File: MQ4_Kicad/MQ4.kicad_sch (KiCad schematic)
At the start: 7 parts, among them J1 Motor_2, J2 Motor_4, J3 Motor_1, J4 Motor_3, J6 Battery_input, U5 LD1117S33TR_SOT223

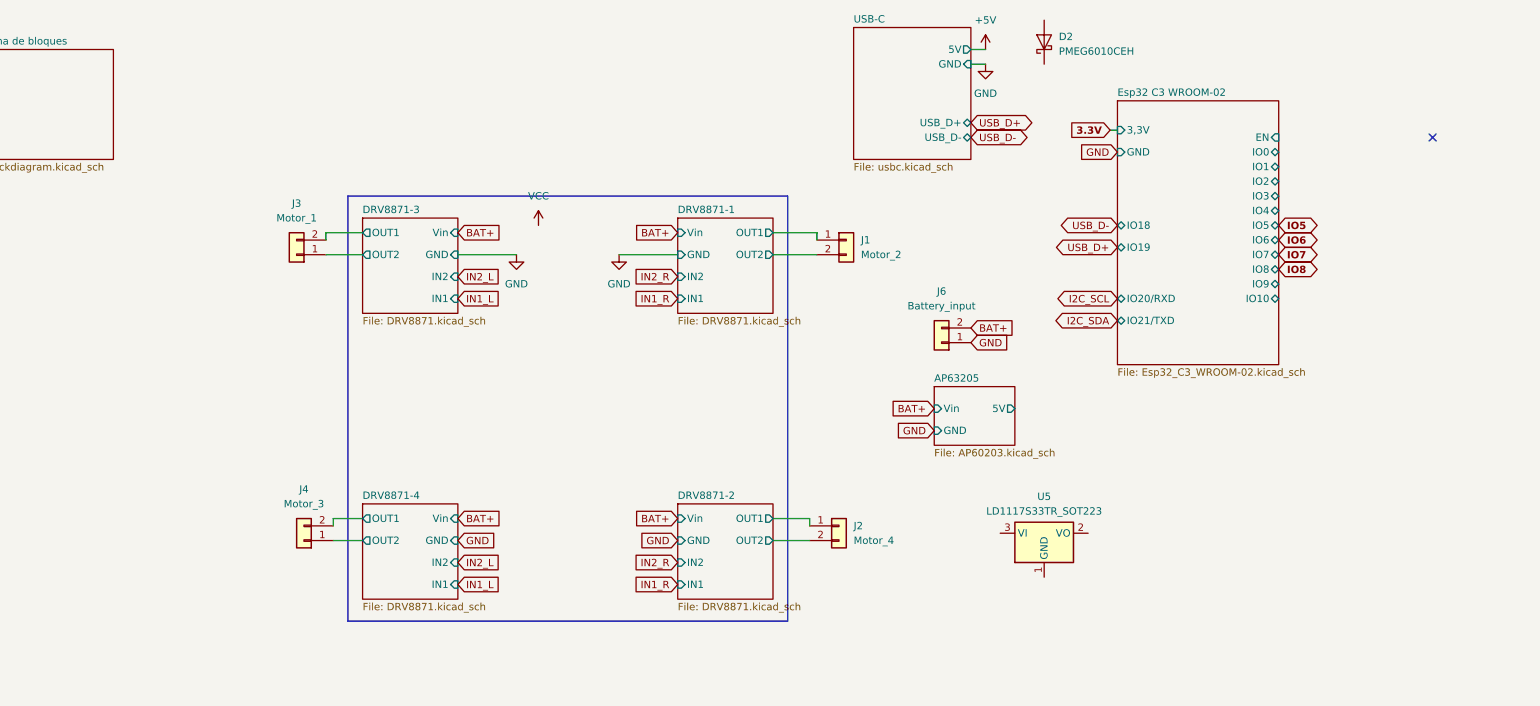
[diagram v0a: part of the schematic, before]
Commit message: Ajustes
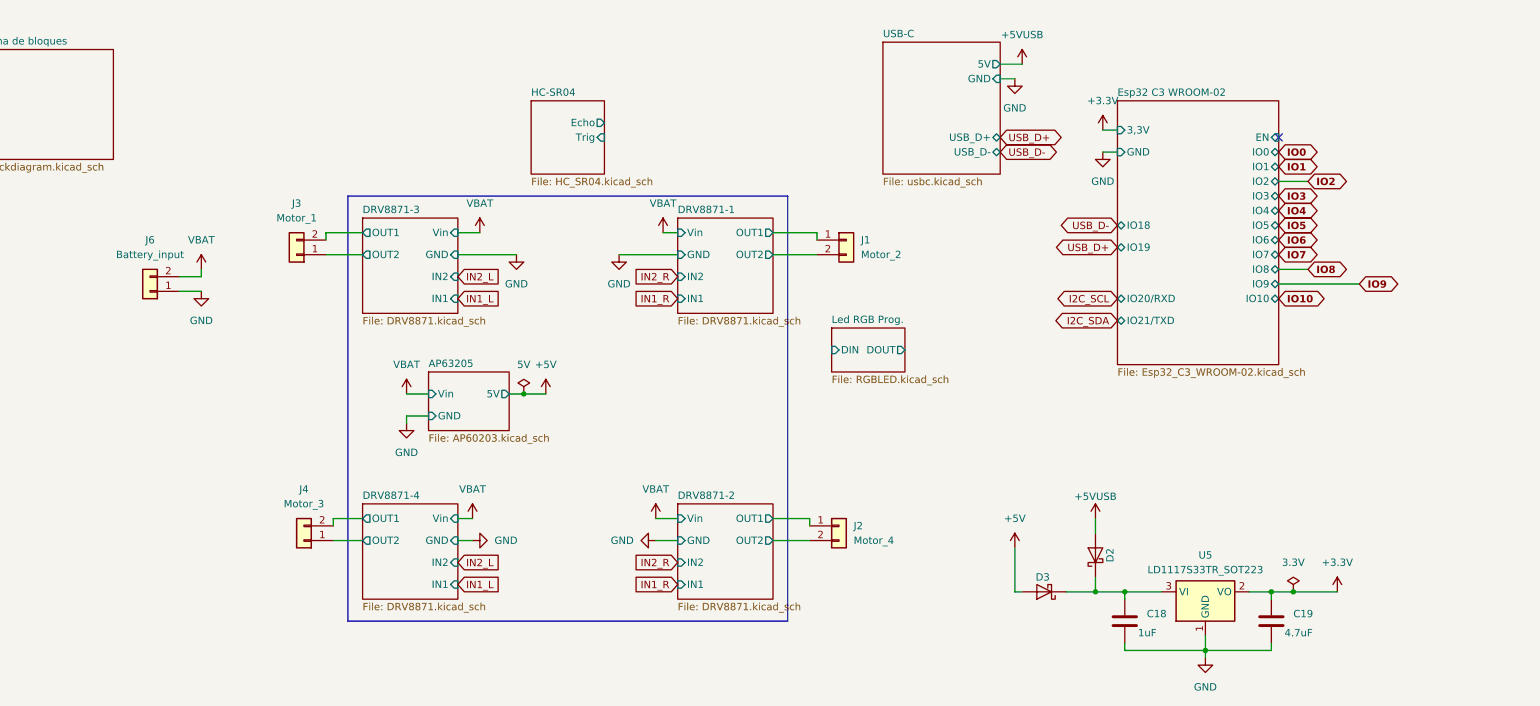
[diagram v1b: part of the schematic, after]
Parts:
- added C18: 1uF, Capacitor_SMD:C_0805_2012Metric, symbol Device:C
- added C19: 4.7uF, Capacitor_SMD:C_0805_2012Metric, symbol Device:C
- added D3: SMD22PL, Diode_SMD:D_SOD-123F, symbol Diode:PMEG6010CEH
- D2: value PMEG6010CEH -> SMD22PL
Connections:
- net +5V: now also D3.2 (A)
- net GND: now also U5.1 (GND), C18.2, C19.2
- net +3.3V: now reaches U5.2 (VO)
- net +3.3V: now also C19.1
- net at U5.3 (VI): now also D2.1 (K), C18.1, D3.1 (K)
- net +5VUSB: now reaches D2.2 (A)
- net BAT+ renamed VBAT
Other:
- added sheet HC-SR04 (HC_SR04.kicad_sch)
- added sheet Led RGB Prog. (RGBLED.kicad_sch)
- moved on the sheet: D2, J6, U5
